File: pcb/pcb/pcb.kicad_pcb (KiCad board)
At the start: 2 copper layers, 65 x 40 mm, 8 parts

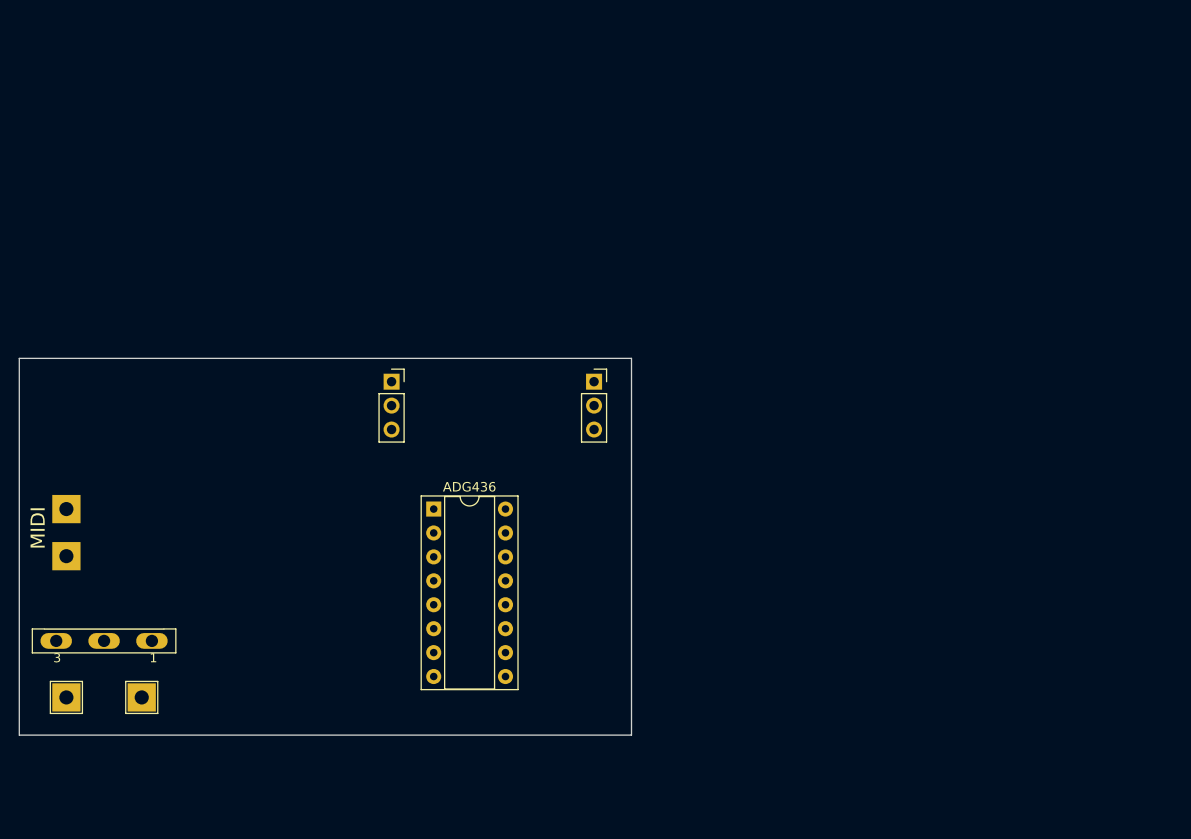
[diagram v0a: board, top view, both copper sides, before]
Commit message: pvb
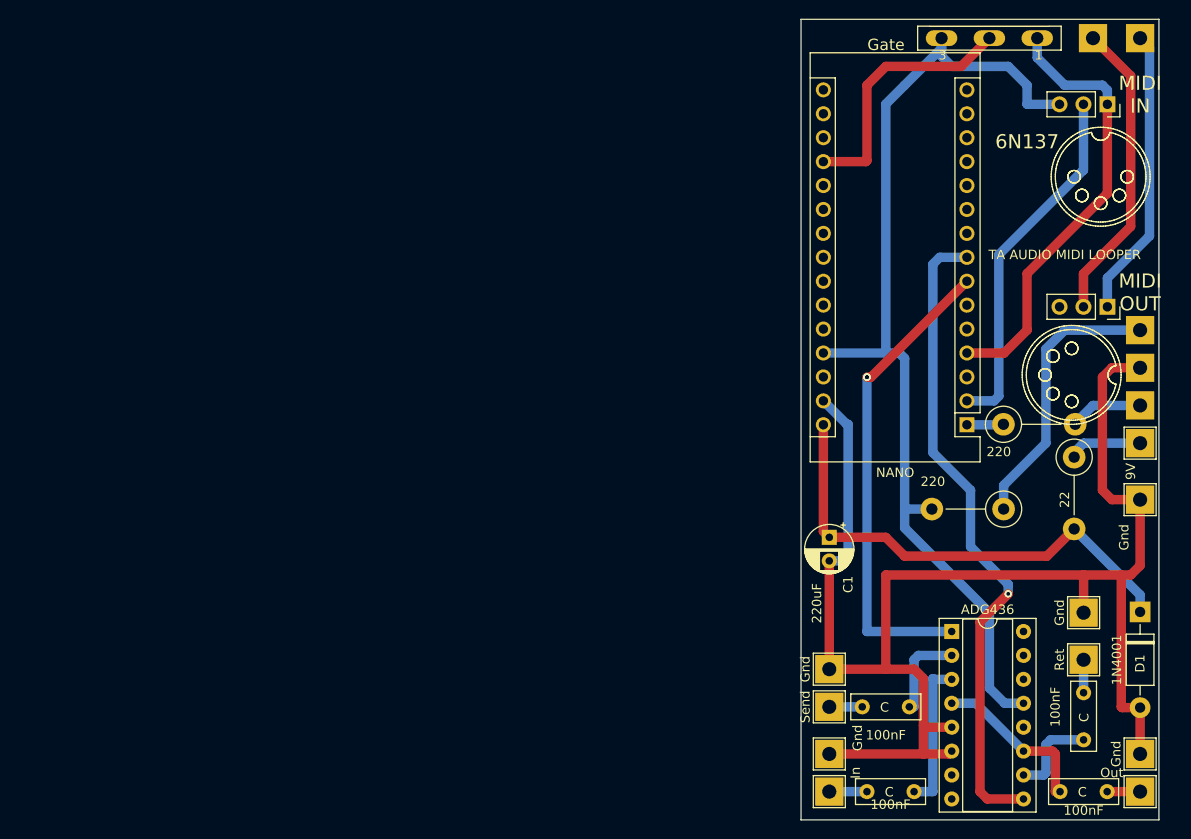
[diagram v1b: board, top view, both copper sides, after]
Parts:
- added ?: 22, Resistor_THT:R_Axial_DIN0411_L9.9mm_D3.6mm_P7.62mm_Vertical, F.Cu at (222.0, 99.5)
- added ?: , , F.Cu at (229.0, 86.0)
- added ?: 220, Resistor_THT:R_Axial_DIN0411_L9.9mm_D3.6mm_P7.62mm_Vertical, F.Cu at (214.5, 105.0)
- added ?: , , F.Cu at (229.0, 94.0)
- added ?: 220, Resistor_THT:R_Axial_DIN0411_L9.9mm_D3.6mm_P7.62mm_Vertical, F.Cu at (214.5, 96.0)
- added ?: , , F.Cu at (229.0, 90.0)
- added C: 100nF, Capacitor_THT:C_Rect_L7.2mm_W2.5mm_P5.00mm_FKS2_FKP2_MKS2_MKP2, F.Cu at (223.0, 124.5)
- added C: 100nF, Capacitor_THT:C_Rect_L7.2mm_W2.5mm_P5.00mm_FKS2_FKP2_MKS2_MKP2, F.Cu at (205.0, 135.0)
- added C: 100nF, Capacitor_THT:C_Rect_L7.2mm_W2.5mm_P5.00mm_FKS2_FKP2_MKS2_MKP2, F.Cu at (204.5, 126.0)
- added C: 100nF, Capacitor_THT:C_Rect_L7.2mm_W2.5mm_P5.00mm_FKS2_FKP2_MKS2_MKP2, F.Cu at (225.5, 135.0)
- added C1: 220uF, Capacitor_THT:CP_Radial_D5.0mm_P2.50mm, F.Cu at (196.0, 108.0)
- added D1: 1N4001, Diode_THT:D_DO-41_SOD81_P10.16mm_Horizontal, F.Cu at (229.0, 115.9)
- added NANO: Arduino_Nano, Module:Arduino_Nano, F.Cu at (210.6, 96.0)
- added REF**: Out, TestPoint:TestPoint_THTPad_3.0x3.0mm_Drill1.5mm, F.Cu at (229.0, 135.0)
- added REF**: Gnd, TestPoint:TestPoint_THTPad_3.0x3.0mm_Drill1.5mm, F.Cu at (229.0, 131.0)
- added REF**: Ret, TestPoint:TestPoint_THTPad_3.0x3.0mm_Drill1.5mm, F.Cu at (223.0, 121.0)
- added REF**: Gnd, TestPoint:TestPoint_THTPad_3.0x3.0mm_Drill1.5mm, F.Cu at (196.0, 122.0)
- added REF**: Send, TestPoint:TestPoint_THTPad_3.0x3.0mm_Drill1.5mm, F.Cu at (196.0, 126.0)
- added REF**: Gnd, TestPoint:TestPoint_THTPad_3.0x3.0mm_Drill1.5mm, F.Cu at (223.0, 116.0)
- added REF**: In, TestPoint:TestPoint_THTPad_3.0x3.0mm_Drill1.5mm, F.Cu at (196.0, 135.0)
- added REF**: Gnd, TestPoint:TestPoint_THTPad_3.0x3.0mm_Drill1.5mm, F.Cu at (196.0, 131.0)
- REF**: value Trim -> Gate
- moved ? 124.5 mm to (229.0, 55.0), turned to -90 degrees
- moved ? 122.1 mm to (224.0, 55.0), turned to -90 degrees
- moved REF** 117.2 mm to (229.0, 98.0), turned to -90 degrees
- moved REF** 113.7 mm to (213.0, 55.0)
- moved REF** 108.1 mm to (229.0, 104.0), turned to -90 degrees
- moved Vcc, Out, Gnd 81.5 mm to (225.5, 62.0), turned to -90 degrees
- moved ADG436 56.5 mm to (209.0, 118.0)
- moved Midi In 55.1 mm to (225.5, 83.5), turned to -90 degrees
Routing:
- net (no net): track 0.00 -> 728.8 mm, vias 0 -> 3
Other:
- board size 65 x 40 mm -> 38 x 85 mm
- board text added: "6N137"
- board text added: "MIDI IN"
- board text added: "MIDI OUT"
- board text added: "TA AUDIO MIDI LOOPER"
- board text removed: "MIDI"
